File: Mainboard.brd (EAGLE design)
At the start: 162.6 x 52.1 mm, 77 parts, among them IC1 MS5611-01BA03, IC2 MCP73831, Q1 BSS84, U1 LM2937IMP-3.3, U2 USD-SOCKETNEW

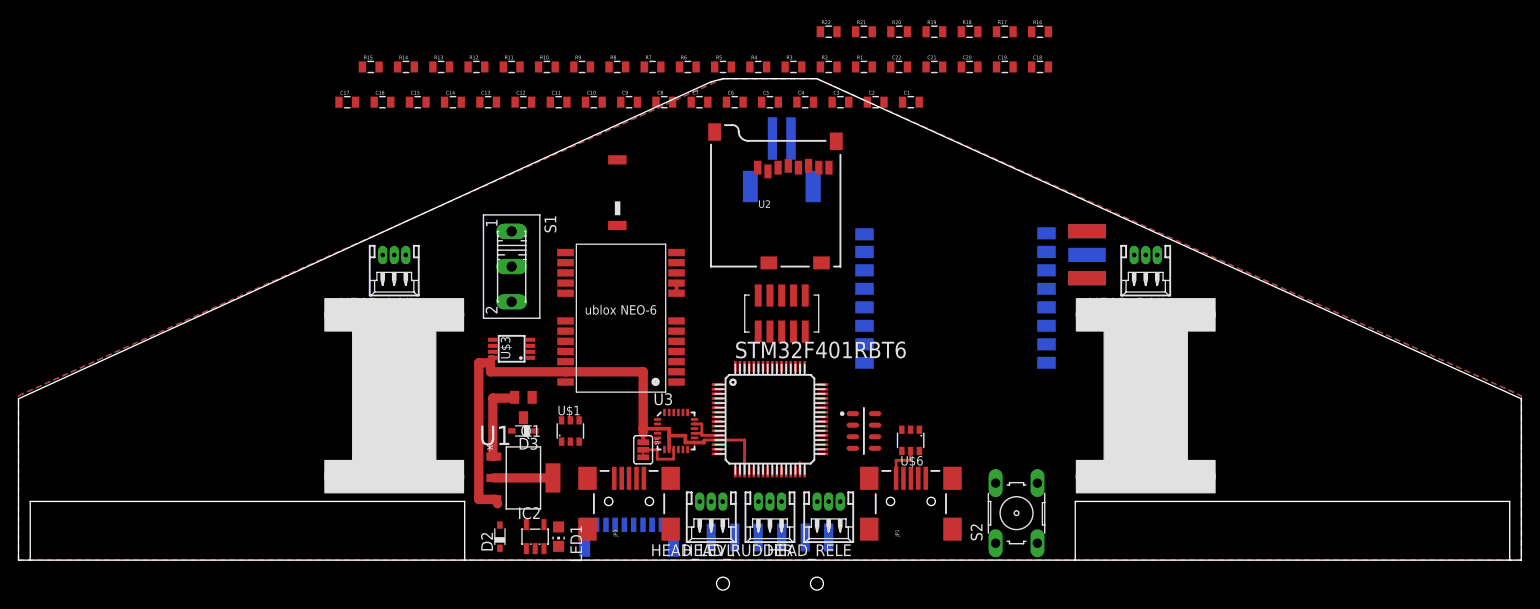
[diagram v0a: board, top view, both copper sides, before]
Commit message: Board rearranged
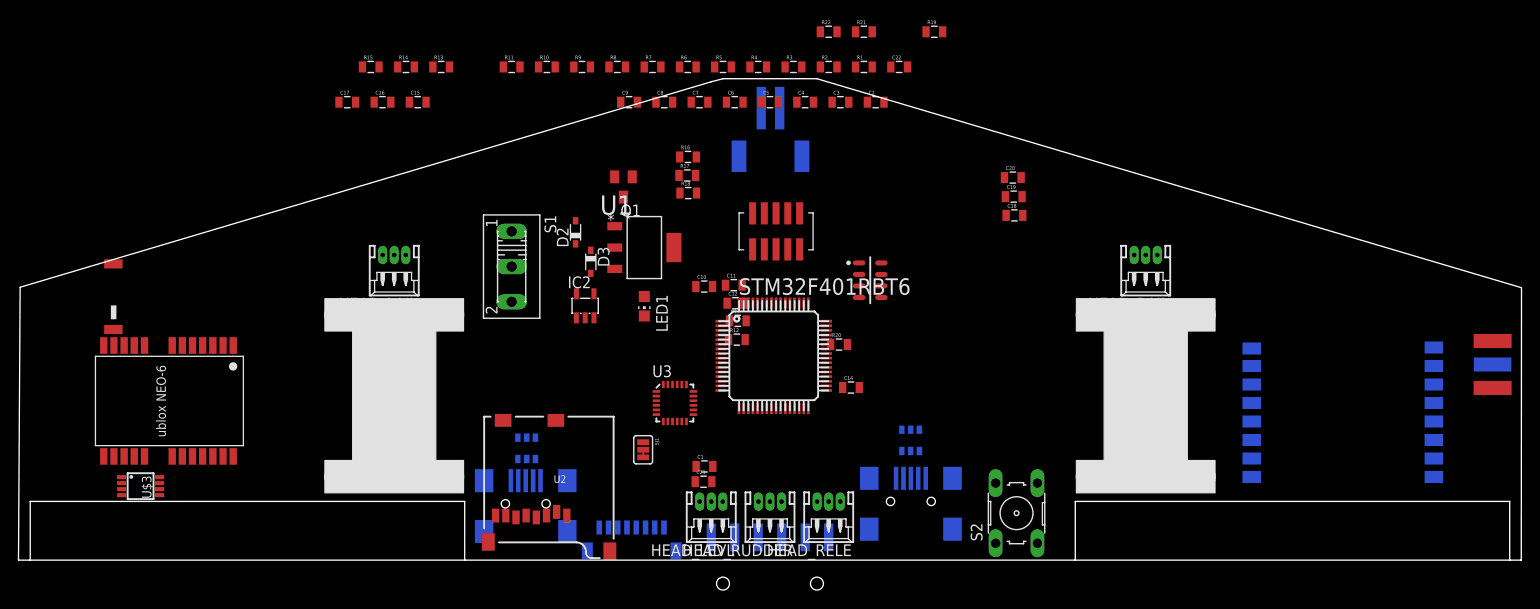
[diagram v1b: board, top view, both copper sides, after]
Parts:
- moved U$4 55.7 mm to (10.3, 40.8)
- moved C14 53.0 mm to (90.0, 31.4)
- moved C21 51.3 mm to (74.1, 21.2)
- moved U$5 49.9 mm to (15.8, 29.5), turned to 90 degrees
- moved J$1 45.4 mm to (159.4, 31.3)
- moved C1 45.3 mm to (74.2, 22.8)
- moved U$8 43.7 mm to (143.5, 28.3)
- moved U$3 42.8 mm to (13.2, 20.7), turned to 270 degrees
- moved U2 41.8 mm to (50.4, 28.2), turned to 180 degrees
- moved R12 40.8 mm to (77.7, 36.6)
- moved R16 40.4 mm to (72.4, 56.3)
- moved R17 37.7 mm to (72.3, 54.3)
- moved C13 35.9 mm to (77.8, 38.6)
- moved R18 35.1 mm to (72.4, 52.4)
- moved R20 34.5 mm to (88.7, 36.0)
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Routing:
- net VDD: track 61.2 -> 0.00 mm
- net GND: track 11.9 -> 0.00 mm
- net N$13: track 8.86 -> 0.00 mm
- net N$15: track 5.37 -> 0.00 mm
- net N$1: track 4.53 -> 0.00 mm
- net N$30: track 1.10 -> 0.00 mm
- net N$3: track 0.57 -> 0.00 mm
- removed copper zone on layer 1, net GND
- removed copper zone on layer 16, net GND
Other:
- outline, holes or cut-outs redrawn
